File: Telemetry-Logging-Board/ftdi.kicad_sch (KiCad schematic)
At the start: 14 parts, among them P1 USB_C_Plug_USB2.0, U8 FT230XQ

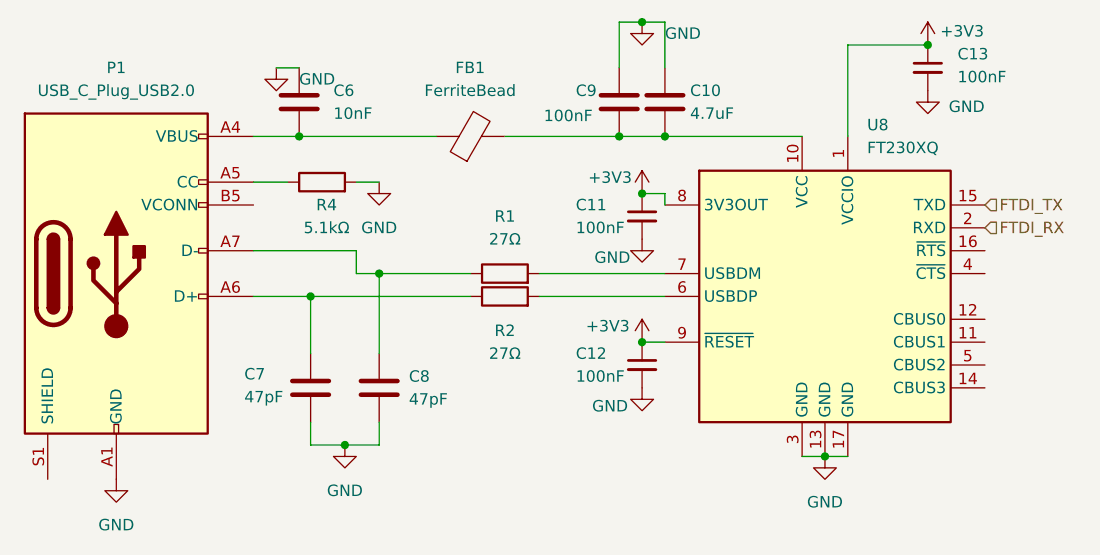
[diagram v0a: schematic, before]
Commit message: varius cleanup, despec audio
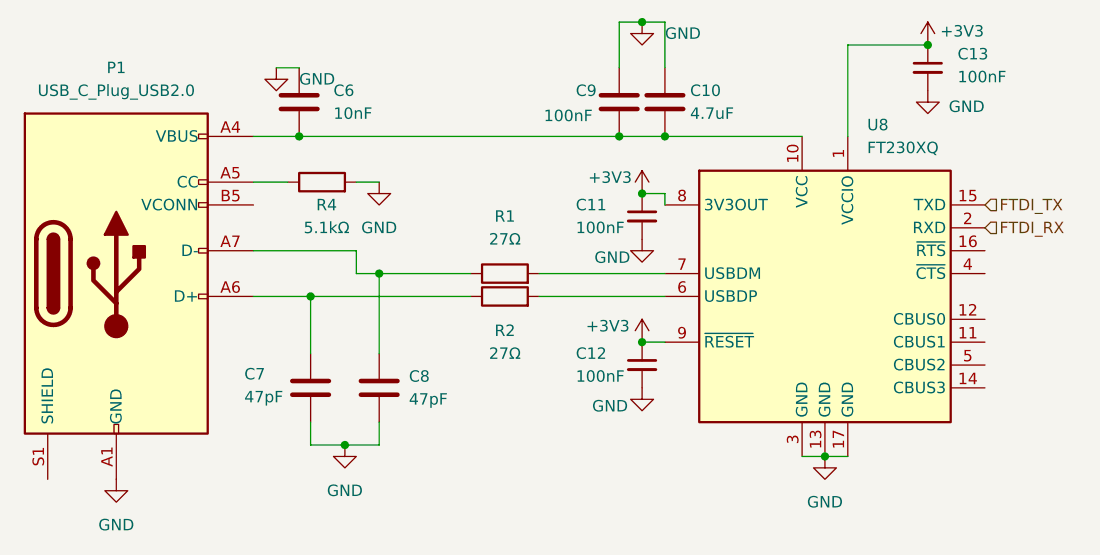
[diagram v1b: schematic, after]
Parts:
- removed FB1: FerriteBead, symbol Device:FerriteBead
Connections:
- net at C6.2, P1.A4 (VBUS), P1.A9 (VBUS)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: now also C10.2, C9.2, U8.10 (VCC)
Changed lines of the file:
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@@
 	(wire
 		(pts
-			(xy 107.95 71.12) (xy 123.19 71.12)
+			(xy 107.95 71.12) (xy 143.51 71.12)
 		)
 		(stroke
@@
 		(pts
 			(xy 166.37 106.68) (xy 168.91 106.68)
-		)
-		(stroke
-			(width 0)
-			(type default)
-		)
-	)
-	(wire
-		(pts
-			(xy 130.81 71.12) (xy 143.51 71.12)
 		)
 		(stroke
@@
 					(unit 1)
 				)
-			)
-		)
-	)
-	(symbol
-		(lib_id "Device:FerriteBead")
-		(at 127 71.12 90)
-		(unit 1)
-		(exclude_from_sim no)
-		(in_bom yes)
-		(on_board yes)
-		(dnp no)
-		(fields_autoplaced yes)
-		(property "Reference" "FB1"
-			(at 126.9492 63.5 90)
-			(effects
-				(font
-					(size 1.27 1.27)
-				)
-			)
-		)
-		(property "Value" "FerriteBead"
-			(at 126.9492 66.04 90)
-			(effects
-				(font
-					(size 1.27 1.27)
-				)
-			)
-		)
-		(property "Footprint" ""
-			(at 127 72.898 90)
-			(effects
-				(font
-					(size 1.27 1.27)
-				)
-				(hide yes)
-			)
-		)
-		(property "Datasheet" "~"
-			(at 127 71.12 0)
-			(effects
-				(font
-					(size 1.27 1.27)
-				)
-				(hide yes)
-			)
-		)
-		(property "Description" "Ferrite bead"
-			(at 127 71.12 0)
-			(effects
-				(font
-					(size 1.27 1.27)
-				)
-				(hide yes)
-			)
-		)
-		(pin "2"
-		)
-		(pin "1"
-		)
-		(instances
-			(project ""
-				(path "/5c64cdbc-39cd-49c8-9a12-12e4867a5d0b/09aa2675-e127-459f-bbca-5f705be2e41d"
-					(reference "FB1")
-					(unit 1)
-				)
